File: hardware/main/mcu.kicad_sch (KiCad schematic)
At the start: 15 parts, among them Q9 SSM3J338R, U1 Holyiot-18010-NRF52840

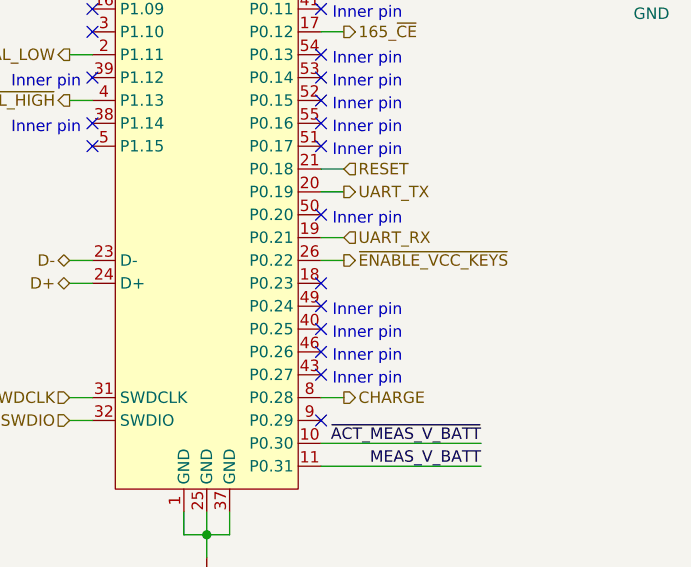
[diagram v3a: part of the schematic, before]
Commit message: Re-add USB voltage sense circuit
Due to firmware limitations the USB voltage cannot be used directly for
waking up the microcontroller.
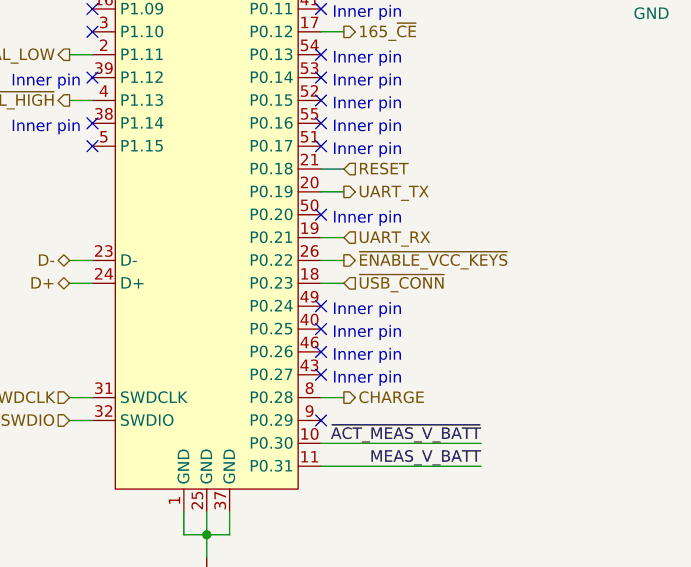
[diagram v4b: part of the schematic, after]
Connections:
- net ~USB_CONN: now reaches U1.18 (P0.23)
- no-connect marks 24 -> 23
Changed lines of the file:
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@@
   (no_connect (at 152.4 87.63))
   (no_connect (at 152.4 95.25))
-  (no_connect (at 152.4 102.87))
   (no_connect (at 152.4 105.41))
   (no_connect (at 152.4 107.95))
@@
     (stroke (width 0) (type solid) (color 0 0 0 0))
   )
+  (wire (pts (xy 152.4 102.87) (xy 154.94 102.87))
+    (stroke (width 0) (type solid) (color 0 0 0 0))
+  )
   (wire (pts (xy 152.4 115.57) (xy 154.94 115.57))
     (stroke (width 0) (type solid) (color 0 0 0 0))
@@
     (effects (font (size 1.27 1.27)) (justify left))
   )
+  (hierarchical_label "~USB_CONN" (shape input) (at 154.94 102.87 0)
+    (effects (font (size 1.27 1.27)) (justify left))
+  )

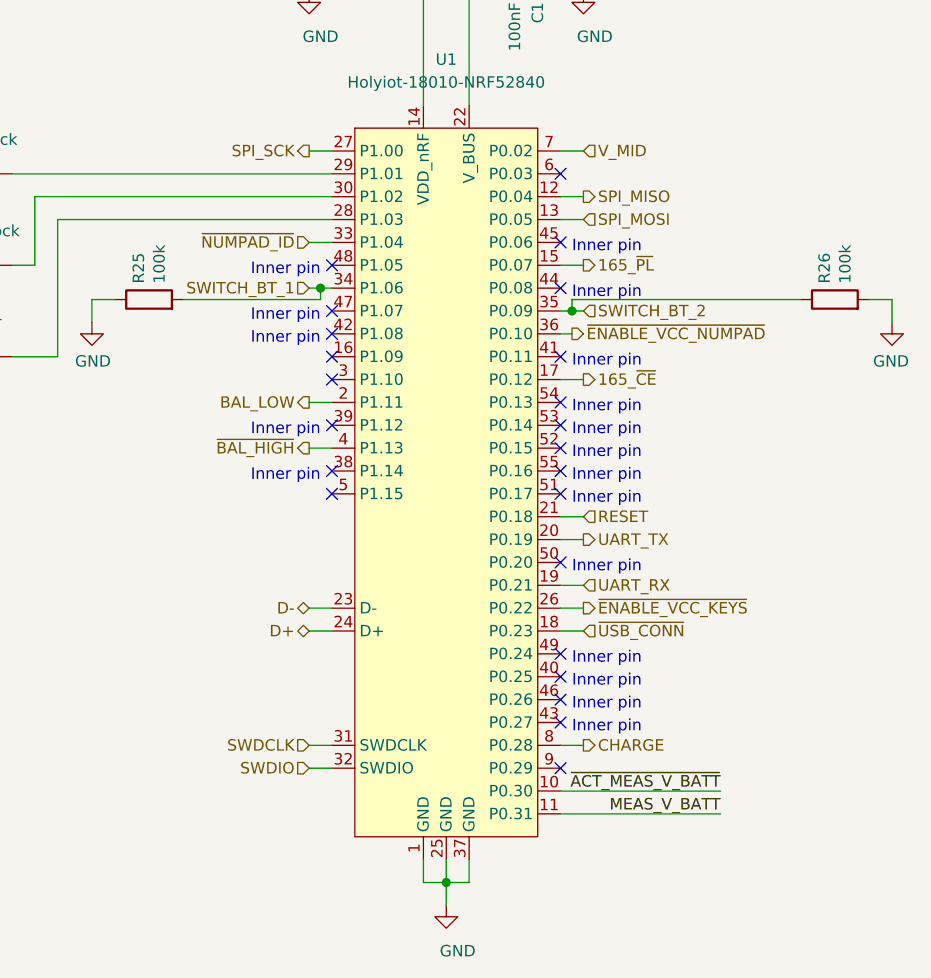
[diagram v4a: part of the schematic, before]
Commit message: Add header with debug pins
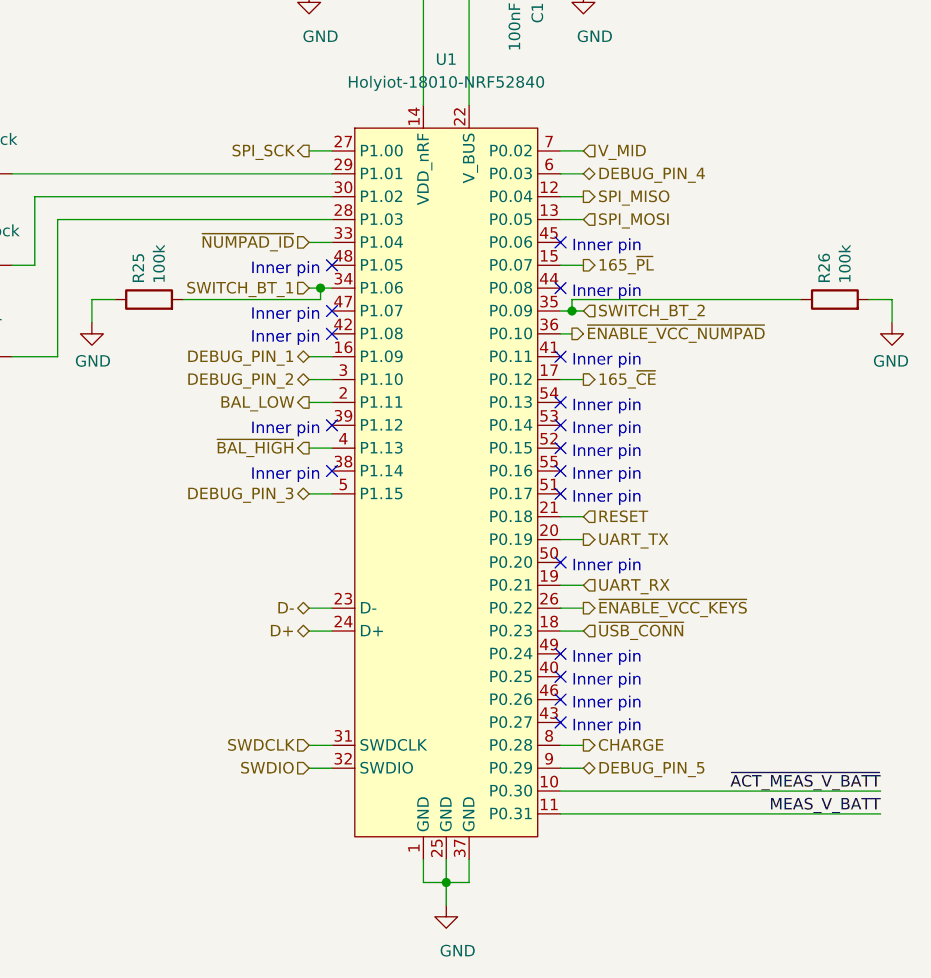
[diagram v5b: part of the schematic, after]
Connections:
- net DEBUG_PIN_1: now reaches U1.16 (P1.09)
- net DEBUG_PIN_2: now reaches U1.3 (P1.10)
- net DEBUG_PIN_3: now reaches U1.5 (P1.15)
- net DEBUG_PIN_4: now reaches U1.6 (P0.03)
- net DEBUG_PIN_5: now reaches U1.9 (P0.29)
- no-connect marks 23 -> 18
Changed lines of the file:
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@@
   (no_connect (at 127 67.31))
   (no_connect (at 127 69.85))
-  (no_connect (at 127 72.39))
-  (no_connect (at 127 74.93))
   (no_connect (at 127 80.01))
   (no_connect (at 127 85.09))
-  (no_connect (at 127 87.63))
-  (no_connect (at 152.4 52.07))
   (no_connect (at 152.4 59.69))
   (no_connect (at 152.4 64.77))
@@
   (no_connect (at 152.4 110.49))
   (no_connect (at 152.4 113.03))
-  (no_connect (at 152.4 118.11))
   (wire (pts (xy 20.32 151.13) (xy 41.91 151.13))
     (stroke (width 0) (type solid) (color 0 0 0 0))
@@
     (stroke (width 0) (type solid) (color 0 0 0 0))
   )
+  (wire (pts (xy 124.46 72.39) (xy 127 72.39))
+    (stroke (width 0) (type solid) (color 0 0 0 0))
+  )
+  (wire (pts (xy 124.46 74.93) (xy 127 74.93))
+    (stroke (width 0) (type solid) (color 0 0 0 0))
+  )
   (wire (pts (xy 124.46 77.47) (xy 127 77.47))
     (stroke (width 0) (type solid) (color 0 0 0 0))
@@
     (stroke (width 0) (type solid) (color 0 0 0 0))
   )
+  (wire (pts (xy 124.46 87.63) (xy 127 87.63))
+    (stroke (width 0) (type solid) (color 0 0 0 0))
+  )
   (wire (pts (xy 124.46 100.33) (xy 127 100.33))
     (stroke (width 0) (type solid) (color 0 0 0 0))
@@
     (stroke (width 0) (type solid) (color 0 0 0 0))
   )
+  (wire (pts (xy 152.4 52.07) (xy 154.94 52.07))
+    (stroke (width 0) (type solid) (color 0 0 0 0))
+  )
   (wire (pts (xy 152.4 54.61) (xy 154.94 54.61))
     (stroke (width 0) (type solid) (color 0 0 0 0))
@@
     (stroke (width 0) (type solid) (color 0 0 0 0))
   )
-  (wire (pts (xy 152.4 120.65) (xy 170.18 120.65))
-    (stroke (width 0) (type solid) (color 0 0 0 0))
-  )
-  (wire (pts (xy 152.4 123.19) (xy 170.18 123.19))
+  (wire (pts (xy 152.4 118.11) (xy 154.94 118.11))
+    (stroke (width 0) (type solid) (color 0 0 0 0))
+  )
+  (wire (pts (xy 152.4 120.65) (xy 187.96 120.65))
+    (stroke (width 0) (type solid) (color 0 0 0 0))
+  )
+  (wire (pts (xy 152.4 123.19) (xy 187.96 123.19))
     (stroke (width 0) (type solid) (color 0 0 0 0))
   )
@@
     (effects (font (size 1.27 1.27)) (justify right bottom))
   )
-  (label "~ACT_MEAS_V_BATT" (at 170.18 120.65 180)
-    (effects (font (size 1.27 1.27)) (justify right bottom))
-  )
-  (label "MEAS_V_BATT" (at 170.18 123.19 180)
+  (label "~ACT_MEAS_V_BATT" (at 187.96 120.65 180)
+    (effects (font (size 1.27 1.27)) (justify right bottom))
+  )
+  (label "MEAS_V_BATT" (at 187.96 123.19 180)
     (effects (font (size 1.27 1.27)) (justify right bottom))
   )
@@
     (effects (font (size 1.27 1.27)) (justify right))
   )
+  (hierarchical_label "DEBUG_PIN_1" (shape bidirectional) (at 124.46 72.39 180)
+    (effects (font (size 1.27 1.27)) (justify right))
+  )
+  (hierarchical_label "DEBUG_PIN_2" (shape bidirectional) (at 124.46 74.93 180)
+    (effects (font (size 1.27 1.27)) (justify right))
+  )
   (hierarchical_label "BAL_LOW" (shape output) (at 124.46 77.47 180)
     (effects (font (size 1.27 1.27)) (justify right))
@@
     (effects (font (size 1.27 1.27)) (justify right))
   )
+  (hierarchical_label "DEBUG_PIN_3" (shape bidirectional) (at 124.46 87.63 180)
+    (effects (font (size 1.27 1.27)) (justify right))
+  )
   (hierarchical_label "D-" (shape bidirectional) (at 124.46 100.33 180)
     (effects (font (size 1.27 1.27)) (justify right))
@@
     (effects (font (size 1.27 1.27)) (justify left))
   )
+  (hierarchical_label "DEBUG_PIN_4" (shape bidirectional) (at 154.94 52.07 0)
+    (effects (font (size 1.27 1.27)) (justify left))
+  )
   (hierarchical_label "SPI_MISO" (shape output) (at 154.94 54.61 0)
     (effects (font (size 1.27 1.27)) (justify left))
@@
     (effects (font (size 1.27 1.27)) (justify left))
   )
+  (hierarchical_label "DEBUG_PIN_5" (shape bidirectional) (at 154.94 118.11 0)
+    (effects (font (size 1.27 1.27)) (justify left))
+  )
